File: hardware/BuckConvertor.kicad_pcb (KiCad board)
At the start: 2 copper layers, 40.8 x 20.8 mm, 20 parts, among them U1 MP2303ADN

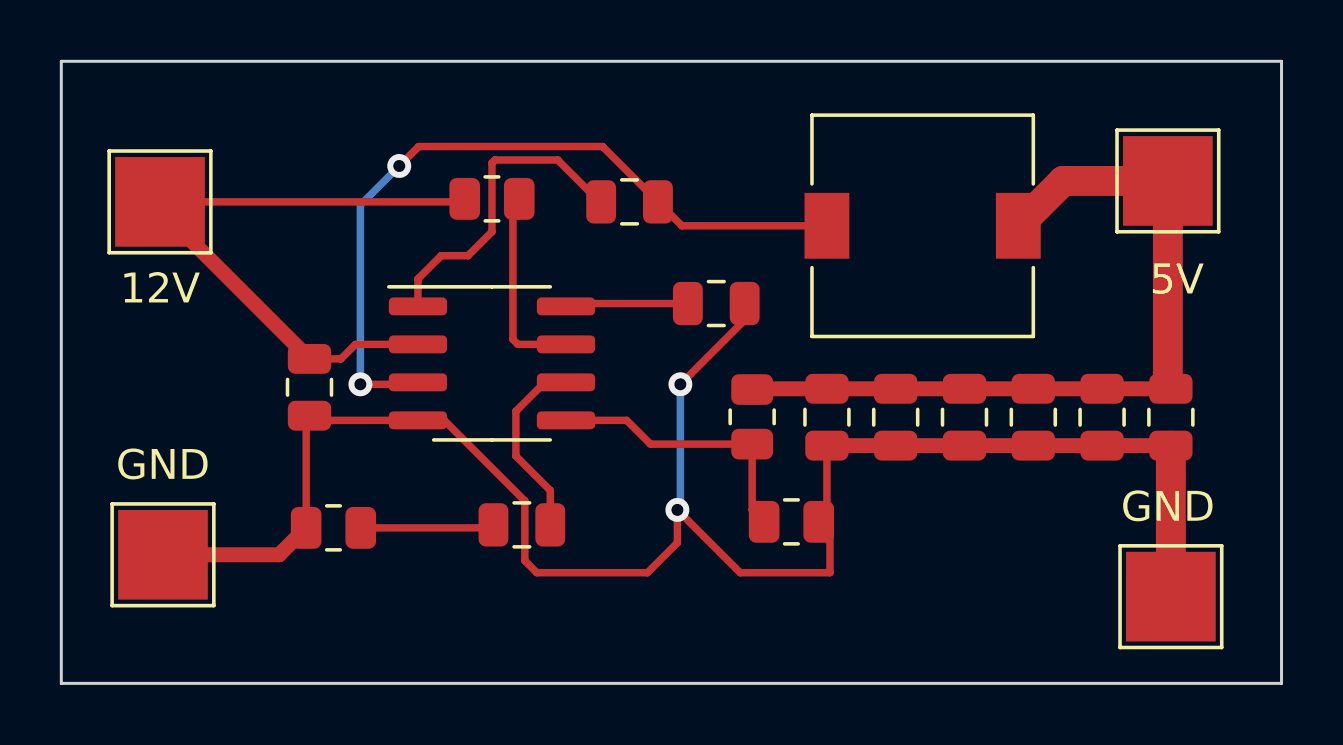
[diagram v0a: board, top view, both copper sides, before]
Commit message: improve version
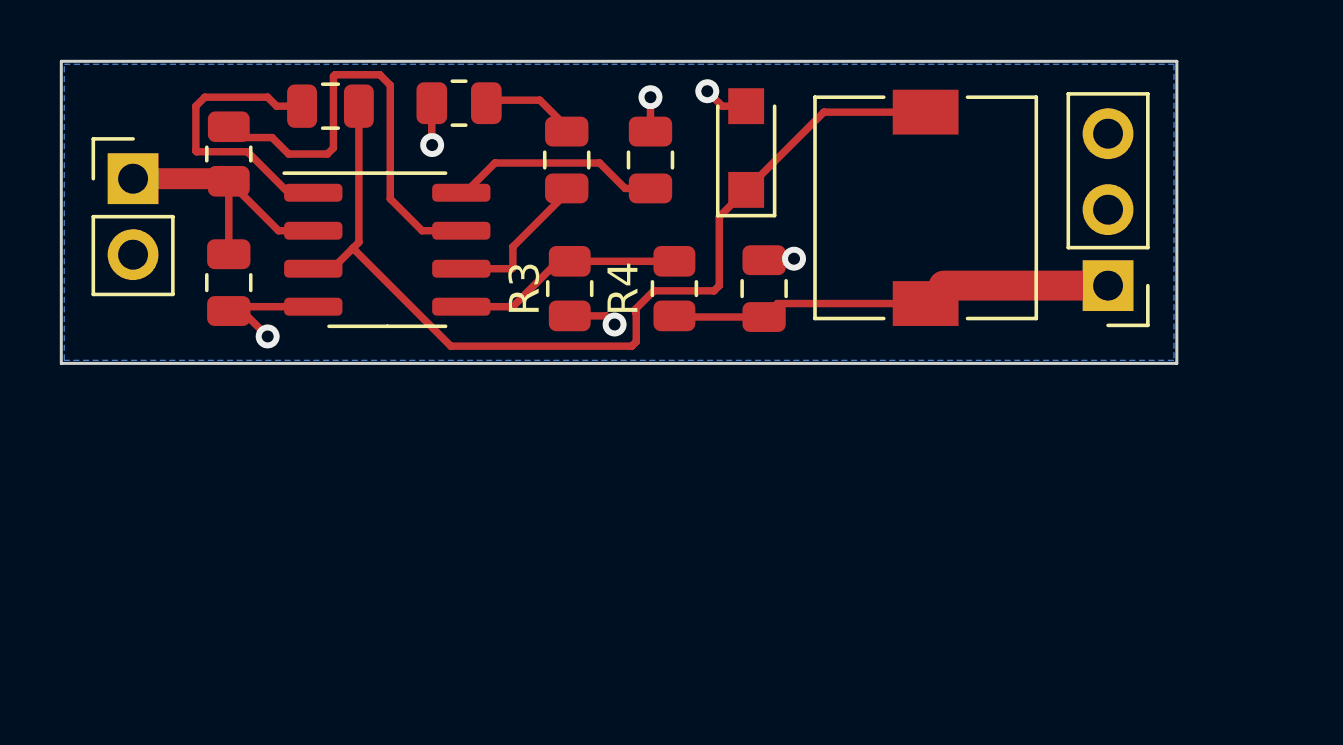
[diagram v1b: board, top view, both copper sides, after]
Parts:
- removed 12V: 12V, TestPoint:TestPoint_Pad_3.0x3.0mm
- removed 5V: 5V, TestPoint:TestPoint_Pad_3.0x3.0mm
- removed C10, C7, C8, C9: 22uF, Capacitor_SMD:C_0805_2012Metric
- removed C3: 10uF, Capacitor_SMD:C_0805_2012Metric
- removed GND (x2): GND, TestPoint:TestPoint_Pad_3.0x3.0mm
- added D1: SS34, Diode_SMD:Nexperia_CFP3_SOD-123W, F.Cu at (158.7, 84.5)
- added J1: INPUT, Connector_PinHeader_2.54mm:PinHeader_1x02_P2.54mm_Vertical, F.Cu at (138.2, 85.5)
- added J2: OUTPUT, Connector_PinHeader_2.54mm:PinHeader_1x03_P2.54mm_Vertical, F.Cu at (170.8, 89.1)
- moved C6 22.7 mm to (141.4, 89.0)
- moved R1 14.8 mm to (149.1, 83.0)
- moved C2 12.3 mm to (152.7, 84.9), turned to -90 degrees
- moved R3 10.8 mm to (152.8, 89.2), turned to 90 degrees
- moved C4 10.5 mm to (144.8, 83.1)
- moved R2 8.93 mm to (141.4, 84.7), turned to 90 degrees
- moved C1 5.28 mm to (155.5, 84.9), turned to -90 degrees
- moved U1 5.17 mm to (146.7, 87.9)
- moved R4 5.01 mm to (156.3, 89.2), turned to 90 degrees
- moved C5 4.79 mm to (159.3, 89.2), turned to -90 degrees
- moved L1 0.61 mm to (164.7, 86.5), turned to 90 degrees
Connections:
- C4 pad 1: Net-(C4-Pad1) -> Net-(L1-Pad2)
- C5 pad 2: Net-(C10-Pad2) -> Net-(L1-Pad1)
- C6 pad 2: Net-(C10-Pad2) -> Net-(C6-Pad2)
- L1 pad 1: Net-(C4-Pad1) -> Net-(L1-Pad1)
- L1 pad 2: Net-(C10-Pad2) -> Net-(L1-Pad2)
- R2 pad 1: Net-(C3-Pad1) -> Net-(C6-Pad2)
- R4 pad 1: Net-(C10-Pad2) -> Net-(L1-Pad1)
- U1 pad 2: Net-(C3-Pad1) -> Net-(C6-Pad2)
- U1 pad 3: Net-(C4-Pad1) -> Net-(L1-Pad2)
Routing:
- net GND: track 61.0 -> 11.2 mm, vias 2 -> 6
- net Net-(L1-Pad2): track 0.00 -> 32.2 mm
- net Net-(C10-Pad2): track 26.6 -> 0.00 mm
- net Net-(C4-Pad1): track 25.5 -> 0.00 mm, vias 2 -> 0
- net Net-(C3-Pad1): track 21.4 -> 0.00 mm
- net Net-(L1-Pad1): track 0.00 -> 14.1 mm
- net Net-(C6-Pad2): track 0.00 -> 9.18 mm
- net Net-(R2-Pad2): track 6.63 -> 15.0 mm
- net Net-(U1-Pad8): track 4.11 -> 7.09 mm
- net Net-(R4-Pad2): track 9.32 -> 7.75 mm
- net Net-(R1-Pad2): track 4.48 -> 3.25 mm
- net Net-(U1-Pad6): track 6.35 -> 5.14 mm
- net Net-(C4-Pad2): track 10.6 -> 9.80 mm
- added copper zone on B.Cu, net GND
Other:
- board size 40.8 x 20.8 mm -> 37.3 x 10.1 mm
- board text added: "Voltage Out = 0.925 * ( R3 + R4 ) / R3 ex. 0.925 * ( 44.2 + 10 ) / 10 = 5.01v"
